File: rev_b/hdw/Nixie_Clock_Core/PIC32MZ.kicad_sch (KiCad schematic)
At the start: 3 parts

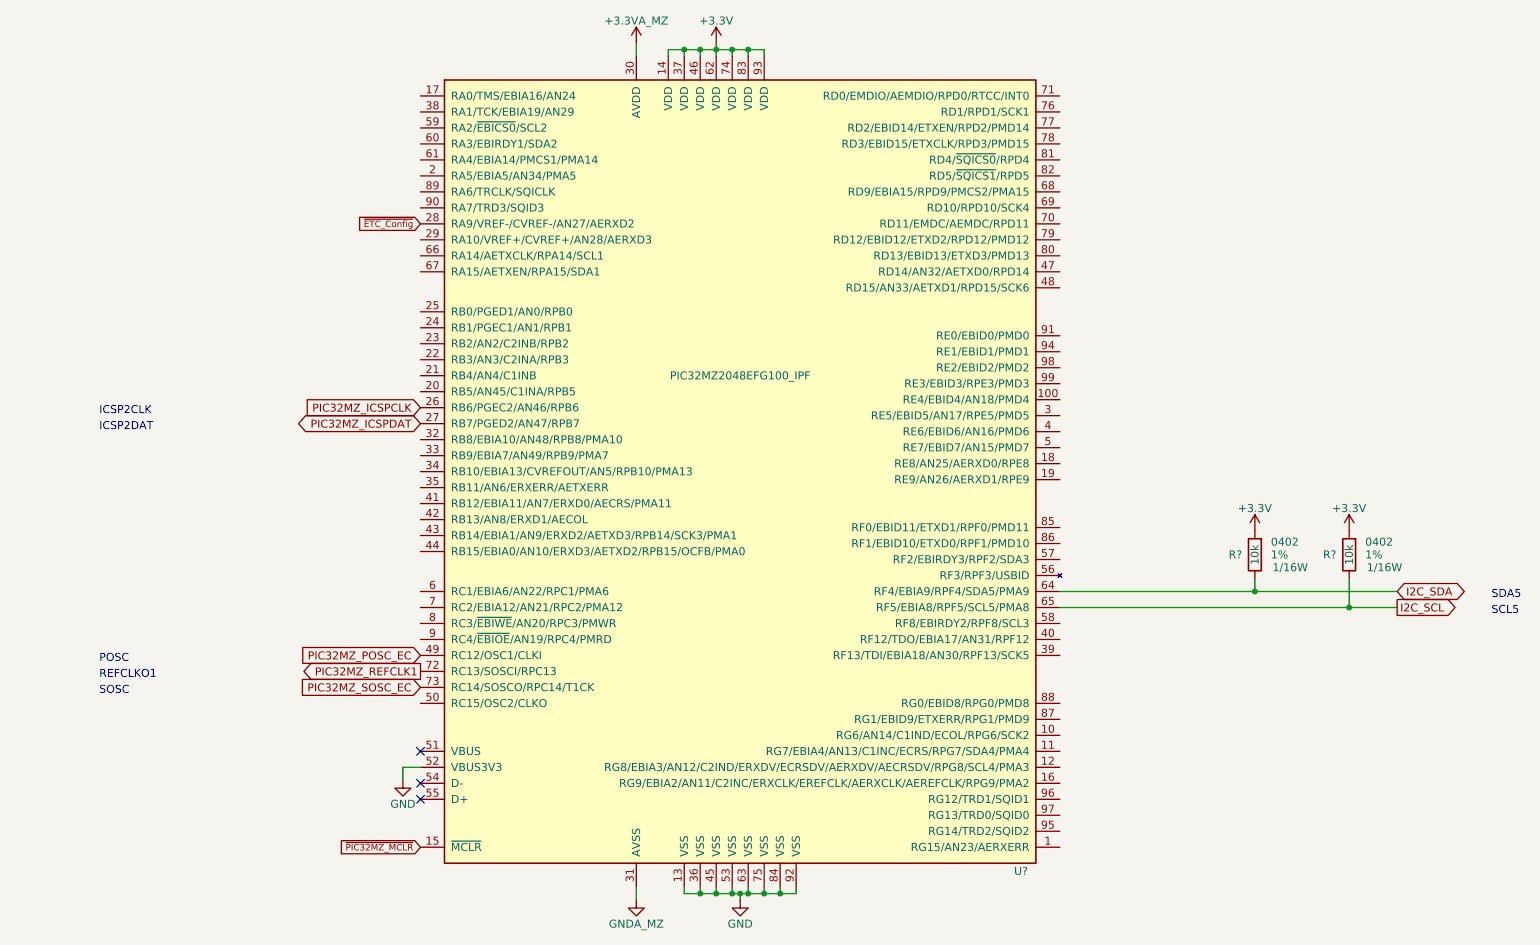
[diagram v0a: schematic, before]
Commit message: more carrier board progress
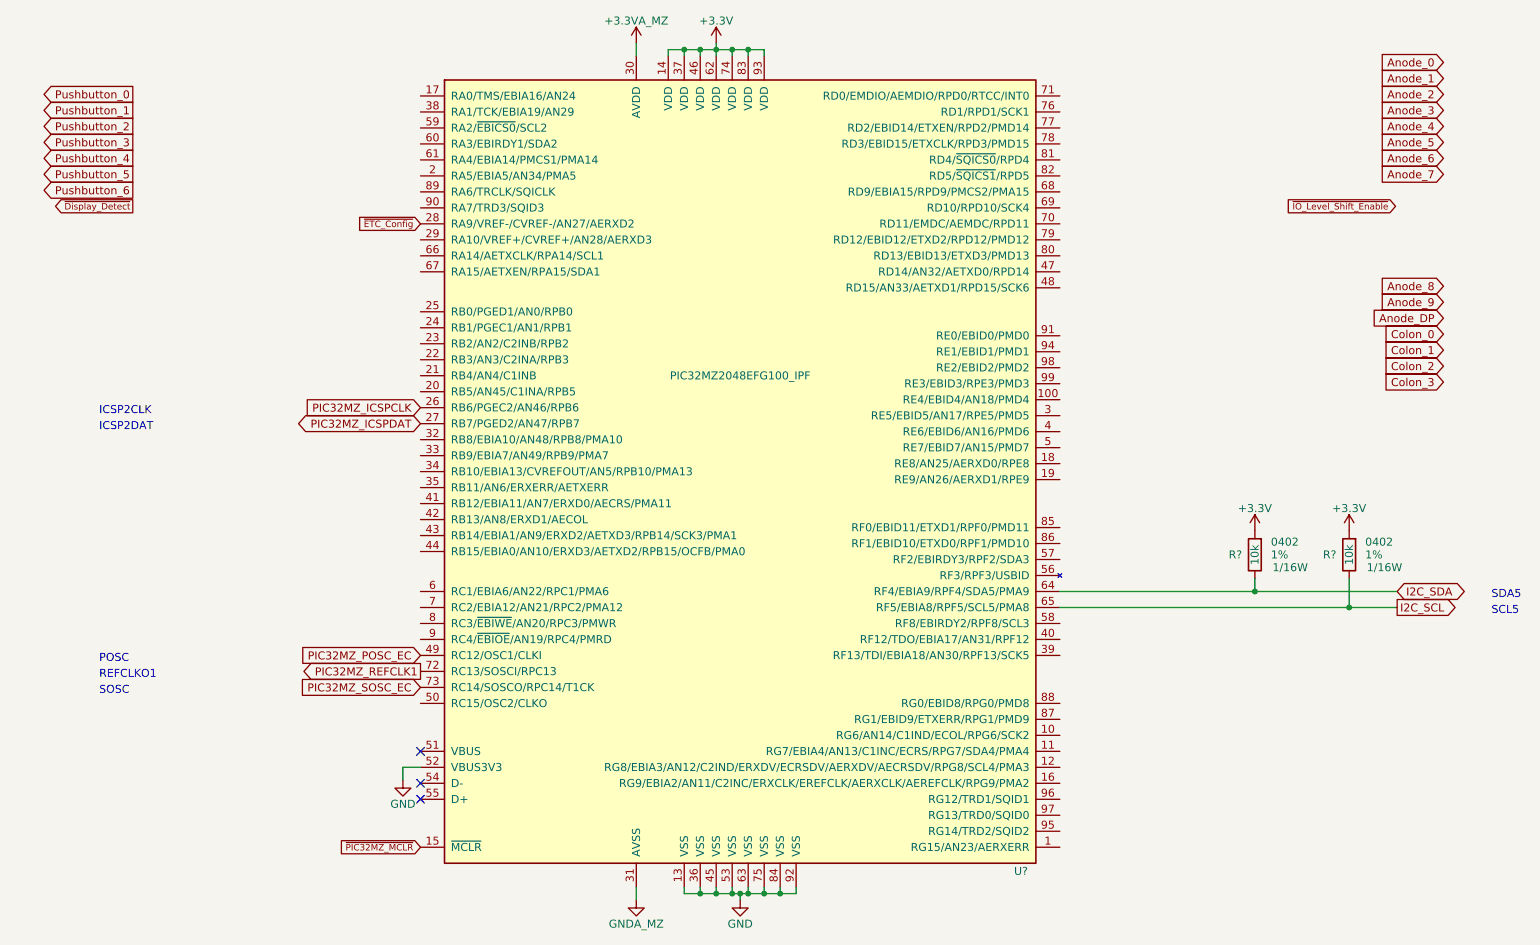
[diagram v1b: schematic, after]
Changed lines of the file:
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@@
+    )
+  )
+  (global_label "Anode_1" (shape input) (at 241.3 27.94 180)
+    (effects (font (size 1.27 1.27)) (justify right))
+    (property "Intersheetrefs" "${INTERSHEET_REFS}" (at 241.3 27.94 0)
+      (effects (font (size 1.27 1.27)) hide)
+    )
+  )
+  (global_label "Pushbutton_4" (shape output) (at 33.02 40.64 180) (fields_autoplaced)
+    (effects (font (size 1.27 1.27)) (justify right))
+    (property "Intersheetrefs" "${INTERSHEET_REFS}" (at 17.2936 40.64 0)
+      (effects (font (size 1.27 1.27)) (justify right) hide)
+    )
+  )
+  (global_label "Anode_5" (shape input) (at 241.3 38.1 180)
+    (effects (font (size 1.27 1.27)) (justify right))
+    (property "Intersheetrefs" "${INTERSHEET_REFS}" (at 241.3 38.1 0)
+      (effects (font (size 1.27 1.27)) hide)
     )
   )
@@
     (effects (font (size 1.27 1.27)) (justify right))
     (property "Intersheetrefs" "${INTERSHEET_REFS}" (at 78.74 124.714 0)
+      (effects (font (size 1.27 1.27)) hide)
+    )
+  )
+  (global_label "Anode_4" (shape input) (at 241.3 35.56 180)
+    (effects (font (size 1.27 1.27)) (justify right))
+    (property "Intersheetrefs" "${INTERSHEET_REFS}" (at 241.3 35.56 0)
+      (effects (font (size 1.27 1.27)) hide)
+    )
+  )
+  (global_label "Pushbutton_6" (shape output) (at 33.02 45.72 180) (fields_autoplaced)
+    (effects (font (size 1.27 1.27)) (justify right))
+    (property "Intersheetrefs" "${INTERSHEET_REFS}" (at 17.2936 45.72 0)
+      (effects (font (size 1.27 1.27)) (justify right) hide)
+    )
+  )
+  (global_label "~{Display_Detect}" (shape output) (at 33.02 48.26 180)
+    (effects (font (size 1.016 1.016)) (justify right))
+    (property "Intersheetrefs" "${INTERSHEET_REFS}" (at 33.02 48.26 0)
       (effects (font (size 1.27 1.27)) hide)
     )
@@
     )
   )
+  (global_label "Colon_1" (shape input) (at 241.3 71.12 180)
+    (effects (font (size 1.27 1.27)) (justify right))
+    (property "Intersheetrefs" "${INTERSHEET_REFS}" (at 241.3 71.12 0)
+      (effects (font (size 1.27 1.27)) hide)
+    )
+  )
+  (global_label "Anode_8" (shape input) (at 241.3 60.96 180)
+    (effects (font (size 1.27 1.27)) (justify right))
+    (property "Intersheetrefs" "${INTERSHEET_REFS}" (at 241.3 60.96 0)
+      (effects (font (size 1.27 1.27)) hide)
+    )
+  )
   (global_label "PIC32MZ_REFCLK1" (shape output) (at 78.74 122.174 180)
     (effects (font (size 1.27 1.27)) (justify right))
     (property "Intersheetrefs" "${INTERSHEET_REFS}" (at 78.74 122.174 0)
+      (effects (font (size 1.27 1.27)) hide)
+    )
+  )
+  (global_label "Anode_7" (shape input) (at 241.3 43.18 180)
+    (effects (font (size 1.27 1.27)) (justify right))
+    (property "Intersheetrefs" "${INTERSHEET_REFS}" (at 241.3 43.18 0)
       (effects (font (size 1.27 1.27)) hide)
     )
@@
     )
   )
+  (global_label "~{IO_Level_Shift_Enable}" (shape input) (at 233.68 48.26 180)
+    (effects (font (size 1.016 1.016)) (justify right))
+    (property "Intersheetrefs" "${INTERSHEET_REFS}" (at 233.68 48.26 0)
+      (effects (font (size 1.27 1.27)) hide)
+    )
+  )
+  (global_label "Anode_3" (shape input) (at 241.3 33.02 180)
+    (effects (font (size 1.27 1.27)) (justify right))
+    (property "Intersheetrefs" "${INTERSHEET_REFS}" (at 241.3 33.02 0)
+      (effects (font (size 1.27 1.27)) hide)
+    )
+  )
   (global_label "~{ETC_Config}" (shape input) (at 78.74 51.054 180)
     (effects (font (size 1.016 1.016)) (justify right))
     (property "Intersheetrefs" "${INTERSHEET_REFS}" (at 78.74 51.054 0)
+      (effects (font (size 1.27 1.27)) hide)
+    )
+  )
+  (global_label "Colon_2" (shape input) (at 241.3 73.66 180)
+    (effects (font (size 1.27 1.27)) (justify right))
+    (property "Intersheetrefs" "${INTERSHEET_REFS}" (at 241.3 73.66 0)
+      (effects (font (size 1.27 1.27)) hide)
+    )
+  )
+  (global_label "Pushbutton_1" (shape output) (at 33.02 33.02 180) (fields_autoplaced)
+    (effects (font (size 1.27 1.27)) (justify right))
+    (property "Intersheetrefs" "${INTERSHEET_REFS}" (at 17.2936 33.02 0)
+      (effects (font (size 1.27 1.27)) (justify right) hide)
+    )
+  )
+  (global_label "Anode_6" (shape input) (at 241.3 40.64 180)
+    (effects (font (size 1.27 1.27)) (justify right))
+    (property "Intersheetrefs" "${INTERSHEET_REFS}" (at 241.3 40.64 0)
       (effects (font (size 1.27 1.27)) hide)
     )
@@
     )
   )
+  (global_label "Pushbutton_5" (shape output) (at 33.02 43.18 180) (fields_autoplaced)
+    (effects (font (size 1.27 1.27)) (justify right))
+    (property "Intersheetrefs" "${INTERSHEET_REFS}" (at 17.2936 43.18 0)
+      (effects (font (size 1.27 1.27)) (justify right) hide)
+    )
+  )
+  (global_label "Pushbutton_0" (shape output) (at 33.02 30.48 180) (fields_autoplaced)
+    (effects (font (size 1.27 1.27)) (justify right))
+    (property "Intersheetrefs" "${INTERSHEET_REFS}" (at 17.2936 30.48 0)
+      (effects (font (size 1.27 1.27)) (justify right) hide)
+    )
+  )
+  (global_label "Pushbutton_2" (shape output) (at 33.02 35.56 180) (fields_autoplaced)
+    (effects (font (size 1.27 1.27)) (justify right))
+    (property "Intersheetrefs" "${INTERSHEET_REFS}" (at 17.2936 35.56 0)
+      (effects (font (size 1.27 1.27)) (justify right) hide)
+    )
+  )
+  (global_label "Colon_3" (shape input) (at 241.3 76.2 180)
+    (effects (font (size 1.27 1.27)) (justify right))
+    (property "Intersheetrefs" "${INTERSHEET_REFS}" (at 241.3 76.2 0)
+      (effects (font (size 1.27 1.27)) hide)
+    )
+  )
+  (global_label "Colon_0" (shape input) (at 241.3 68.58 180)
+    (effects (font (size 1.27 1.27)) (justify right))
+    (property "Intersheetrefs" "${INTERSHEET_REFS}" (at 241.3 68.58 0)
+      (effects (font (size 1.27 1.27)) hide)
+    )
+  )
+  (global_label "Pushbutton_3" (shape output) (at 33.02 38.1 180) (fields_autoplaced)
+    (effects (font (size 1.27 1.27)) (justify right))
+    (property "Intersheetrefs" "${INTERSHEET_REFS}" (at 17.2936 38.1 0)
+      (effects (font (size 1.27 1.27)) (justify right) hide)
+    )
+  )
   (global_label "I2C_SCL" (shape output) (at 233.934 112.014 0)
     (effects (font (size 1.27 1.27)) (justify left))
@@
       (effects (font (size 1.27 1.27)) hide)
     )
+  )
+  (global_label "Anode_2" (shape input) (at 241.3 30.48 180)
+    (effects (font (size 1.27 1.27)) (justify right))
+    (property "Intersheetrefs" "${INTERSHEET_REFS}" (at 241.3 30.48 0)
+      (effects (font (size 1.27 1.27)) hide)
+    )
+  )
+  (global_label "Anode_0" (shape input) (at 241.3 25.4 180)
+    (effects (font (size 1.27 1.27)) (justify right))
+    (property "Intersheetrefs" "${INTERSHEET_REFS}" (at 241.3 25.4 0)
+      (effects (font (size 1.27 1.27)) hide)
+    )
+  )
+  (global_label "Anode_DP" (shape input) (at 241.3 66.04 180)
+    (effects (font (size 1.27 1.27)) (justify right))
+    (property "Intersheetrefs" "${INTERSHEET_REFS}" (at 241.3 66.04 0)
+      (effects (font (size 1.27 1.27)) hide)
+    )
+  )
+  (global_label "Anode_9" (shape input) (at 241.3 63.5 180)
+    (effects (font (size 1.27 1.27)) (justify right))
+    (property "Intersheetrefs" "${INTERSHEET_REFS}" (at 241.3 63.5 0)
+      (effects (font (size 1.27 1.27)) hide)
+    )
